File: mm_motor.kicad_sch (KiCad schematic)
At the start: 1 part, among them M1 N20_encoder

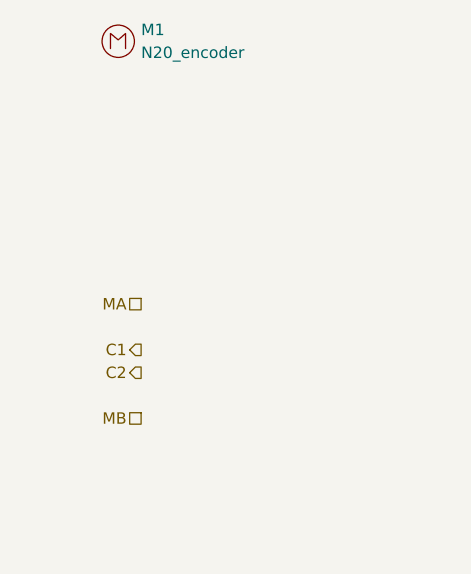
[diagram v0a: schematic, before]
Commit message: tp2
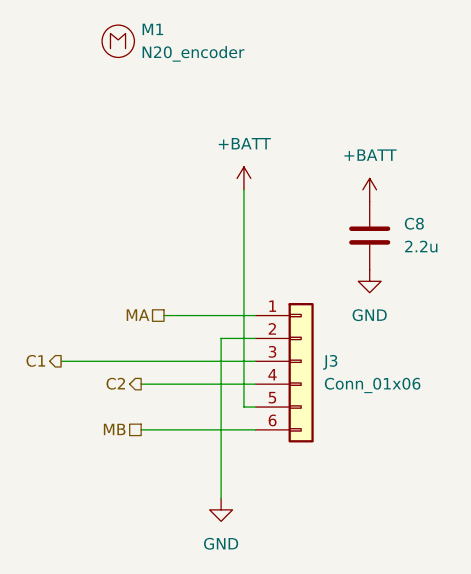
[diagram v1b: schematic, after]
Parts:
- added C8: 2.2u, symbol Device:C
- added J3: Conn_01x06, symbol Connector_Generic:Conn_01x06
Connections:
- net C1: now also J3.3 (Pin_3)
- net C2: now also J3.4 (Pin_4)
- net MA: now also J3.1 (Pin_1)
- net MB: now also J3.6 (Pin_6)
- new net +BATT: C8.1, J3.5 (Pin_5)
- new net GND: C8.2, J3.2 (Pin_2)
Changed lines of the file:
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@@
 (kicad_sch (version 20230121) (generator eeschema)
   (paper "A4")
-  (hierarchical_label "C1" (shape output) (at 118.11 91.44 180) (fields_autoplaced)
-    (effects (font (size 1.27 1.27)) (justify right))
-  )
-  (hierarchical_label "C2" (shape output) (at 118.11 93.98 180) (fields_autoplaced)
-    (effects (font (size 1.27 1.27)) (justify right))
-  )
-  (hierarchical_label "MB" (shape passive) (at 118.11 99.06 180) (fields_autoplaced)
-    (effects (font (size 1.27 1.27)) (justify right))
-  )
-  (hierarchical_label "MA" (shape passive) (at 118.11 86.36 180) (fields_autoplaced)
-    (effects (font (size 1.27 1.27)) (justify right))
+  (wire (pts (xy 129.54 97.79) (xy 130.81 97.79))
+    (stroke (width 0) (type default))
+  )
+  (wire (pts (xy 130.81 87.63) (xy 120.65 87.63))
+    (stroke (width 0) (type default))
+  )
+  (wire (pts (xy 127 90.17) (xy 127 107.95))
+    (stroke (width 0) (type default))
+  )
+  (wire (pts (xy 127 90.17) (xy 130.81 90.17))
+    (stroke (width 0) (type default))
+  )
+  (wire (pts (xy 118.11 95.25) (xy 130.81 95.25))
+    (stroke (width 0) (type default))
+  )
+  (wire (pts (xy 109.22 92.71) (xy 130.81 92.71))
+    (stroke (width 0) (type default))
+  )
+  (wire (pts (xy 130.81 100.33) (xy 118.11 100.33))
+    (stroke (width 0) (type default))
+  )
+  (wire (pts (xy 129.54 73.66) (xy 129.54 97.79))
+    (stroke (width 0) (type default))
+  )
+  (hierarchical_label "C1" (shape output) (at 109.22 92.71 180) (fields_autoplaced)
+    (effects (font (size 1.27 1.27)) (justify right))
+  )
+  (hierarchical_label "C2" (shape output) (at 118.11 95.25 180) (fields_autoplaced)
+    (effects (font (size 1.27 1.27)) (justify right))
+  )
+  (hierarchical_label "MB" (shape passive) (at 118.11 100.33 180) (fields_autoplaced)
+    (effects (font (size 1.27 1.27)) (justify right))
+  )
+  (hierarchical_label "MA" (shape passive) (at 120.65 87.63 180) (fields_autoplaced)
+    (effects (font (size 1.27 1.27)) (justify right))
+  )
+  (symbol (lib_id "power:GND") (at 143.51 82.55 0) (unit 1)
+    (in_bom yes) (on_board yes) (dnp no) (fields_autoplaced)
+    (property "Reference" "#PWR027" (at 143.51 88.9 0)
+      (effects (font (size 1.27 1.27)) hide)
+    )
+    (property "Value" "GND" (at 143.51 87.63 0)
+      (effects (font (size 1.27 1.27)))
+    )
+    (property "Footprint" "" (at 143.51 82.55 0)
+      (effects (font (size 1.27 1.27)) hide)
+    )
+    (property "Datasheet" "" (at 143.51 82.55 0)
+      (effects (font (size 1.27 1.27)) hide)
+    )
+    (pin "1")
+    (instances
+      (project "minimouse"
+        (path "/d8fa4cba-2469-4231-847f-065b6b829f44/7f113667-692a-4f4d-b16f-621d32f3f136"
+          (reference "#PWR027") (unit 1)
+        )
+        (path "/d8fa4cba-2469-4231-847f-065b6b829f44/3975acd0-18ad-47bc-9ce1-d8c4d864aafe"
+          (reference "#PWR028") (unit 1)
+        )
+      )
+    )
+  )
+  (symbol (lib_id "power:+BATT") (at 143.51 74.93 0) (unit 1)
+    (in_bom yes) (on_board yes) (dnp no) (fields_autoplaced)
+    (property "Reference" "#PWR036" (at 143.51 78.74 0)
+      (effects (font (size 1.27 1.27)) hide)
+    )
+    (property "Value" "+BATT" (at 143.51 69.85 0)
+      (effects (font (size 1.27 1.27)))
+    )
+    (property "Footprint" "" (at 143.51 74.93 0)
+      (effects (font (size 1.27 1.27)) hide)
+    )
+    (property "Datasheet" "" (at 143.51 74.93 0)
+      (effects (font (size 1.27 1.27)) hide)
+    )
+    (pin "1")
+    (instances
+      (project "minimouse"
+        (path "/d8fa4cba-2469-4231-847f-065b6b829f44/3f9b0845-5778-418c-a7a8-03da2392145e"
+          (reference "#PWR036") (unit 1)
+        )
+        (path "/d8fa4cba-2469-4231-847f-065b6b829f44/7f113667-692a-4f4d-b16f-621d32f3f136"
+          (reference "#PWR033") (unit 1)
+        )
+        (path "/d8fa4cba-2469-4231-847f-065b6b829f44/3975acd0-18ad-47bc-9ce1-d8c4d864aafe"
+          (reference "#PWR034") (unit 1)
+        )
+      )
+    )
   )
   (symbol (lib_id "minimouse:N20_w_encoder") (at 115.57 57.15 0) (unit 1)
@@
         )
       )
+    )
+  )
+  (symbol (lib_id "power:+BATT") (at 129.54 73.66 0) (unit 1)
+    (in_bom yes) (on_board yes) (dnp no) (fields_autoplaced)
+    (property "Reference" "#PWR036" (at 129.54 77.47 0)
+      (effects (font (size 1.27 1.27)) hide)
+    )
+    (property "Value" "+BATT" (at 129.54 68.58 0)
+      (effects (font (size 1.27 1.27)))
+    )
+    (property "Footprint" "" (at 129.54 73.66 0)
+      (effects (font (size 1.27 1.27)) hide)
+    )
+    (property "Datasheet" "" (at 129.54 73.66 0)
+      (effects (font (size 1.27 1.27)) hide)
+    )
+    (pin "1")
+    (instances
+      (project "minimouse"
+        (path "/d8fa4cba-2469-4231-847f-065b6b829f44/3f9b0845-5778-418c-a7a8-03da2392145e"
+          (reference "#PWR036") (unit 1)
+        )
+        (path "/d8fa4cba-2469-4231-847f-065b6b829f44/7f113667-692a-4f4d-b16f-621d32f3f136"
+          (reference "#PWR035") (unit 1)
+        )
+        (path "/d8fa4cba-2469-4231-847f-065b6b829f44/3975acd0-18ad-47bc-9ce1-d8c4d864aafe"
+          (reference "#PWR038") (unit 1)
+        )
+      )
+    )
+  )
+  (symbol (lib_id "Connector_Generic:Conn_01x06") (at 135.89 92.71 0) (unit 1)
+    (in_bom yes) (on_board yes) (dnp no) (fields_autoplaced)
+    (property "Reference" "J3" (at 138.43 92.71 0)
+      (effects (font (size 1.27 1.27)) (justify left))
+    )
+    (property "Value" "Conn_01x06" (at 138.43 95.25 0)
+      (effects (font (size 1.27 1.27)) (justify left))
+    )
+    (property "Footprint" "" (at 135.89 92.71 0)
+      (effects (font (size 1.27 1.27)) hide)
+    )
+    (property "Datasheet" "~" (at 135.89 92.71 0)
+      (effects (font (size 1.27 1.27)) hide)
+    )
+    (pin "3")
+    (pin "2")
+    (pin "1")
+    (pin "5")
+    (pin "6")
+    (pin "4")
+    (instances
+      (project "minimouse"
+        (path "/d8fa4cba-2469-4231-847f-065b6b829f44/7f113667-692a-4f4d-b16f-621d32f3f136"
+          (reference "J3") (unit 1)
+        )
+        (path "/d8fa4cba-2469-4231-847f-065b6b829f44/3975acd0-18ad-47bc-9ce1-d8c4d864aafe"
+          (reference "J4") (unit 1)
+        )
+      )
+    )
+  )
+  (symbol (lib_id "power:GND") (at 127 107.95 0) (unit 1)
+    (in_bom yes) (on_board yes) (dnp no) (fields_autoplaced)
+    (property "Reference" "#PWR020" (at 127 114.3 0)
+      (effects (font (size 1.27 1.27)) hide)
+    )
+    (property "Value" "GND" (at 127 113.03 0)
+      (effects (font (size 1.27 1.27)))
+    )
+    (property "Footprint" "" (at 127 107.95 0)
+      (effects (font (size 1.27 1.27)) hide)
+    )
+    (property "Datasheet" "" (at 127 107.95 0)
+      (effects (font (size 1.27 1.27)) hide)
+    )
+    (pin "1")
+    (instances
+      (project "minimouse"
+        (path "/d8fa4cba-2469-4231-847f-065b6b829f44/7f113667-692a-4f4d-b16f-621d32f3f136"
+          (reference "#PWR020") (unit 1)
+        )
+        (path "/d8fa4cba-2469-4231-847f-065b6b829f44/3975acd0-18ad-47bc-9ce1-d8c4d864aafe"
+          (reference "#PWR021") (unit 1)
+        )
+      )
+    )
+  )
+  (symbol (lib_id "Device:C") (at 143.51 78.74 0) (unit 1)
+    (in_bom yes) (on_board yes) (dnp no) (fields_autoplaced)
+    (property "Reference" "C8" (at 147.32 77.47 0)
+      (effects (font (size 1.27 1.27)) (justify left))
+    )
+    (property "Value" "2.2u" (at 147.32 80.01 0)
+      (effects (font (size 1.27 1.27)) (justify left))
+    )
+    (property "Footprint" "" (at 144.4752 82.55 0)
+      (effects (font (size 1.27 1.27)) hide)
+    )
+    (property "Datasheet" "~" (at 143.51 78.74 0)
+      (effects (font (size 1.27 1.27)) hide)
+    )
+    (pin "2")
+    (pin "1")
+    (instances
+      (project "minimouse"
+        (path "/d8fa4cba-2469-4231-847f-065b6b829f44/7f113667-692a-4f4d-b16f-621d32f3f136"
+          (reference "C8") (unit 1)
+        )
+        (path "/d8fa4cba-2469-4231-847f-065b6b829f44/3975acd0-18ad-47bc-9ce1-d8c4d864aafe"
+          (reference "C9") (unit 1)
+        )
+      )
